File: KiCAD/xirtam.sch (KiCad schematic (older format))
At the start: 26 parts, among them J1 To Computer, J2 To Keyboard, J3 Power, J4 JTAG, J5 Bootloader, J6 Debug Serial Port, P1 USB_A, SW1 Reset, U1 MT093APR1, U2 AT90USB1287, Y1 16 MHz

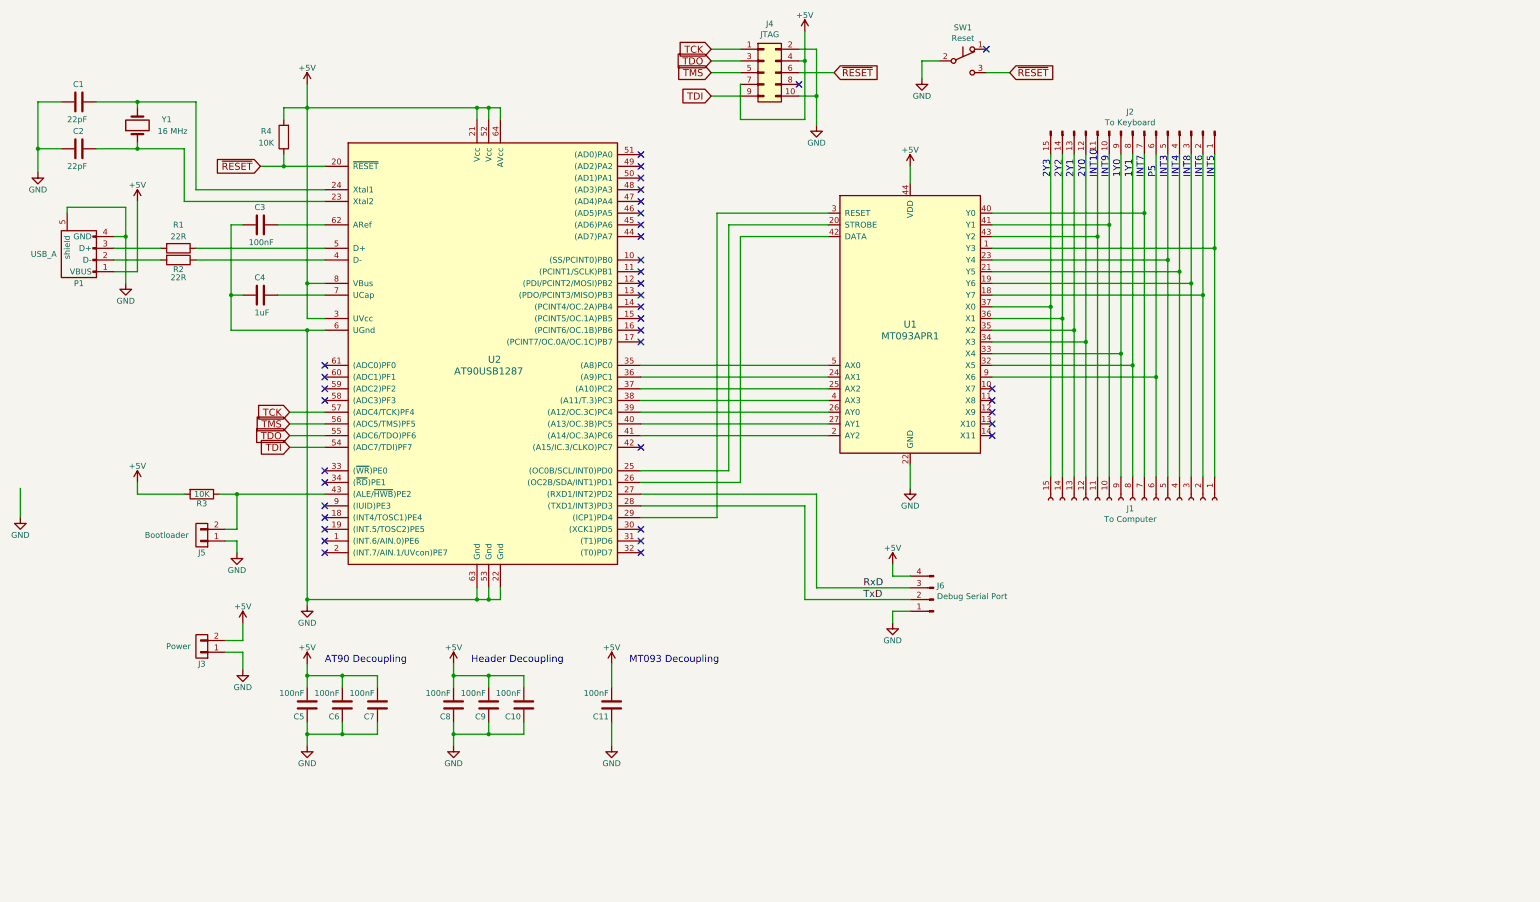
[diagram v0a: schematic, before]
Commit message: New PCB layout
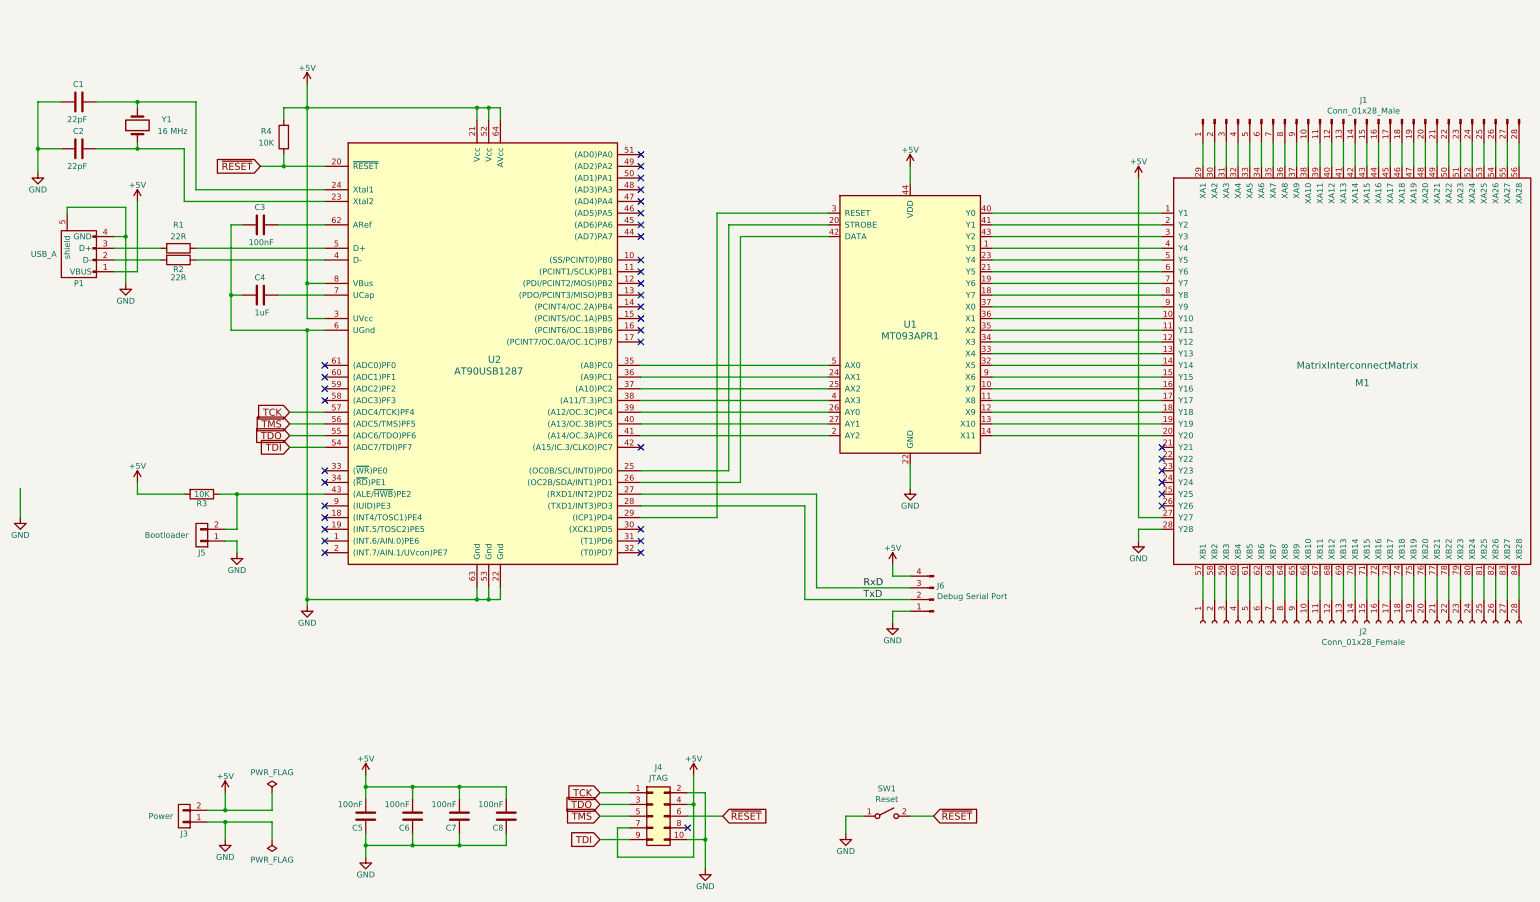
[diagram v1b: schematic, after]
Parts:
- removed C7, C8, C9: 100nF, Capacitor_SMD:C_0603_1608Metric_Pad1.05x0.95mm_HandSolder, symbol Device:C
- removed J1: To Computer, Connector_PinSocket_2.54mm:PinSocket_1x15_P2.54mm_Horizontal, symbol Connector:Conn_01x15_Female
- removed J2: To Keyboard, Connector_PinHeader_2.54mm:PinHeader_1x15_P2.54mm_Horizontal, symbol Connector:Conn_01x15_Male
- removed SW1: Reset, Button_Switch_SMD:SW_Push_1P1T_NO_6x6mm_H9.5mm, symbol Switch:SW_Push_SPDT
- added J1: Conn_01x28_Male, Connector_PinHeader_2.54mm:PinHeader_1x28_P2.54mm_Horizontal, symbol Connector:Conn_01x28_Male
- added J2: Conn_01x28_Female, Connector_PinSocket_2.54mm:PinSocket_1x28_P2.54mm_Horizontal, symbol Connector:Conn_01x28_Female
- added M1: MatrixInterconnectMatrix, Jumper:matrixinterconnectmatrix, symbol Jumper:MatrixInterconnectMatrix
- added SW1: Reset, Button_Switch_SMD:SW_SPST_FSMSM, symbol Switch:SW_SPST
- J6: footprint (none) -> Connector_PinHeader_2.54mm:PinHeader_1x04_P2.54mm_Horizontal
- renumbered C10 to C7, C11 to C8
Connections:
- net +5V: now also M1.27 (Y27)
- net GND: now also M1.28 (Y28), SW1.1 (A)
- net ~RESET: now also SW1.2 (B)
- net at U1.1 (Y3): now also M1.4 (Y4)
- net at U1.10 (X7): now also M1.16 (Y16)
- net at U1.11 (X8): now also M1.17 (Y17)
- net at U1.12 (X9): now also M1.18 (Y18)
- net at U1.13 (X10): now also M1.19 (Y19)
- net at U1.14 (X11): now also M1.20 (Y20)
- net at U1.18 (Y7): now also M1.8 (Y8)
- net at U1.19 (Y6): now also M1.7 (Y7)
- net at U1.21 (Y5): now also M1.6 (Y6)
- net at U1.23 (Y4): now also M1.5 (Y5)
- net at U1.32 (X5): now also M1.14 (Y14)
- net at U1.33 (X4): now also M1.13 (Y13)
- net at U1.34 (X3): now also M1.12 (Y12)
- net at U1.35 (X2): now also M1.11 (Y11)
- net at U1.36 (X1): now also M1.10 (Y10)
- net at U1.37 (X0): now also M1.9 (Y9)
- net at U1.40 (Y0): now also M1.1 (Y1)
- net at U1.41 (Y1): now also M1.2 (Y2)
- net at U1.43 (Y2): now also M1.3 (Y3)
- net at U1.9 (X6): now also M1.15 (Y15)
- new net: J1.1 (Pin_1), M1.29 (XA1)
- new net: J1.2 (Pin_2), M1.30 (XA2)
- new net: J1.3 (Pin_3), M1.31 (XA3)
- new net: J1.4 (Pin_4), M1.32 (XA4)
- new net: J1.5 (Pin_5), M1.33 (XA5)
- new net: J1.6 (Pin_6), M1.34 (XA6)
- new net: J1.7 (Pin_7), M1.35 (XA7)
- new net: J1.8 (Pin_8), M1.36 (XA8)
- new net: J1.9 (Pin_9), M1.37 (XA9)
- new net: J1.10 (Pin_10), M1.38 (XA10)
- new net: J1.11 (Pin_11), M1.39 (XA11)
- new net: J1.12 (Pin_12), M1.40 (XA12)
- new net: J1.13 (Pin_13), M1.41 (XA13)
- new net: J1.14 (Pin_14), M1.42 (XA14)
- new net: J1.15 (Pin_15), M1.43 (XA15)
- new net: J1.16 (Pin_16), M1.44 (XA16)
- new net: J1.17 (Pin_17), M1.45 (XA17)
- new net: J1.18 (Pin_18), M1.46 (XA18)
- new net: J1.19 (Pin_19), M1.47 (XA19)
- new net: J1.20 (Pin_20), M1.48 (XA20)
- new net: J1.21 (Pin_21), M1.49 (XA21)
- new net: J1.22 (Pin_22), M1.50 (XA22)
- new net: J1.23 (Pin_23), M1.51 (XA23)
- new net: J1.24 (Pin_24), M1.52 (XA24)
- new net: J1.25 (Pin_25), M1.53 (XA25)
- new net: J1.26 (Pin_26), M1.54 (XA26)
- new net: J1.27 (Pin_27), M1.55 (XA27)
- new net: J1.28 (Pin_28), M1.56 (XA28)
- new net: J2.1 (Pin_1), M1.57 (XB1)
- new net: J2.2 (Pin_2), M1.58 (XB2)
- new net: J2.3 (Pin_3), M1.59 (XB3)
- new net: J2.4 (Pin_4), M1.60 (XB4)
- new net: J2.5 (Pin_5), M1.61 (XB5)
- new net: J2.6 (Pin_6), M1.62 (XB6)
- new net: J2.7 (Pin_7), M1.63 (XB7)
- new net: J2.8 (Pin_8), M1.64 (XB8)
- new net: J2.9 (Pin_9), M1.65 (XB9)
- new net: J2.10 (Pin_10), M1.66 (XB10)
- new net: J2.11 (Pin_11), M1.67 (XB11)
- new net: J2.12 (Pin_12), M1.68 (XB12)
- new net: J2.13 (Pin_13), M1.69 (XB13)
- new net: J2.14 (Pin_14), M1.70 (XB14)
- new net: J2.15 (Pin_15), M1.71 (XB15)
- new net: J2.16 (Pin_16), M1.72 (XB16)
- new net: J2.17 (Pin_17), M1.73 (XB17)
- new net: J2.18 (Pin_18), M1.74 (XB18)
- new net: J2.19 (Pin_19), M1.75 (XB19)
- new net: J2.20 (Pin_20), M1.76 (XB20)
- new net: J2.21 (Pin_21), M1.77 (XB21)
- new net: J2.22 (Pin_22), M1.78 (XB22)
- new net: J2.23 (Pin_23), M1.79 (XB23)
- new net: J2.24 (Pin_24), M1.80 (XB24)
- new net: J2.25 (Pin_25), M1.81 (XB25)
- new net: J2.26 (Pin_26), M1.82 (XB26)
- new net: J2.27 (Pin_27), M1.83 (XB27)
- new net: J2.28 (Pin_28), M1.84 (XB28)
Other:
- note removed: "1Y0"
- note removed: "1Y1"
- note removed: "2Y0"
- note removed: "2Y1"
- note removed: "2Y2"
- note removed: "2Y3"
- note removed: "AT90 Decoupling"
- note removed: "Header Decoupling"
- note removed: "INT10"
- note removed: "INT3"
- note removed: "INT4"
- note removed: "INT5"
- note removed: "INT6"
- note removed: "INT7"
- note removed: "INT8"
- note removed: "INT9"
- note removed: "MT093 Decoupling"
- note removed: "P5"
- moved on the sheet: C5, C6, C7, C8, J3, J4
